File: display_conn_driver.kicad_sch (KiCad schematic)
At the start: 9 parts, among them IC5 AW9364DNR

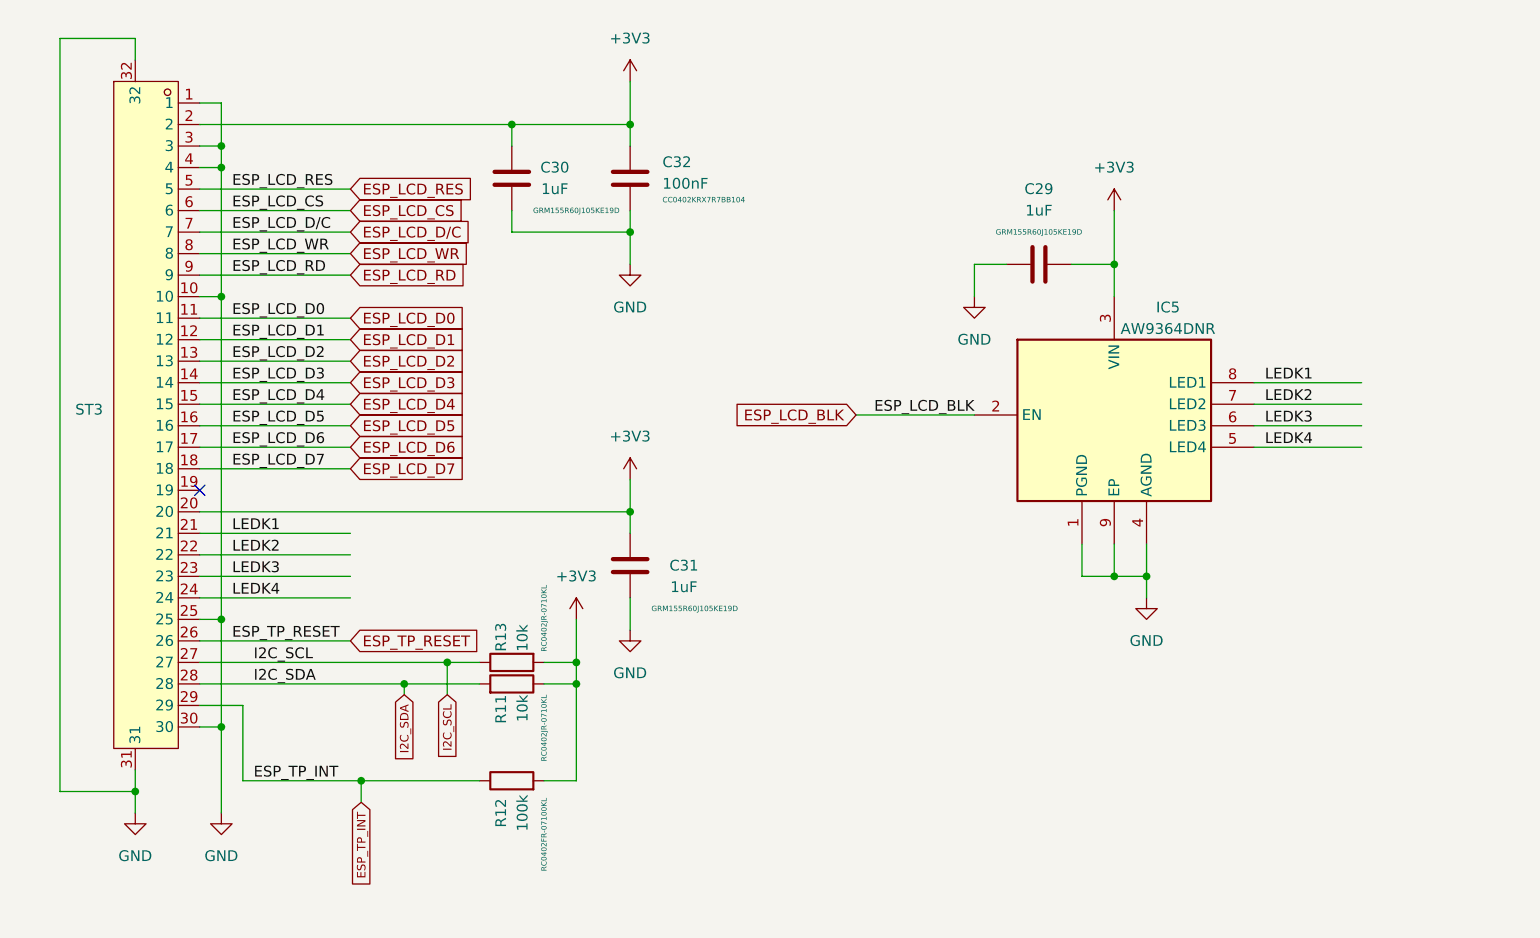
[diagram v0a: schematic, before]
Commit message: Minor changes to styling
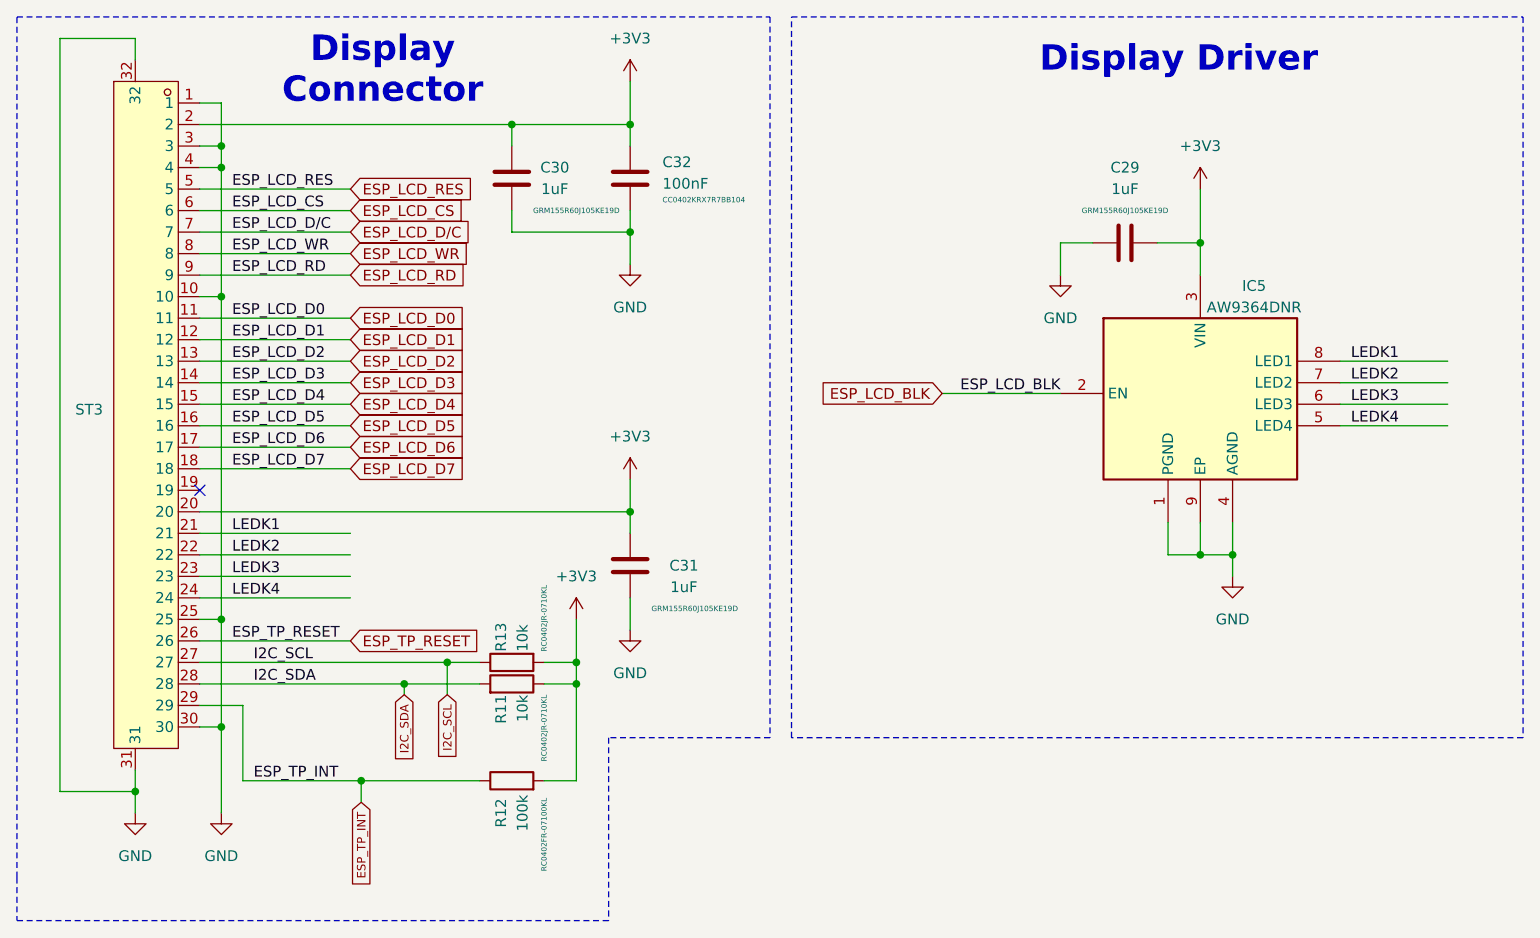
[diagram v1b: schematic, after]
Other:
- note added: "Display Connector"
- note added: "Display Driver"
- moved on the sheet: C29, IC5
